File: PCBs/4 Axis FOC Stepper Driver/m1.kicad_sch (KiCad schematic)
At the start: 3 parts, among them J2 M1

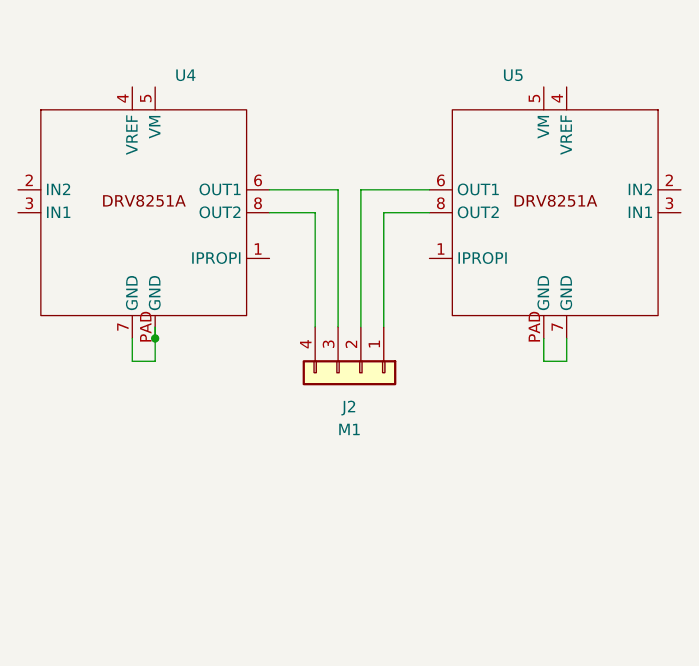
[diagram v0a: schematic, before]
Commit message: Start working on an integrated stepper driver
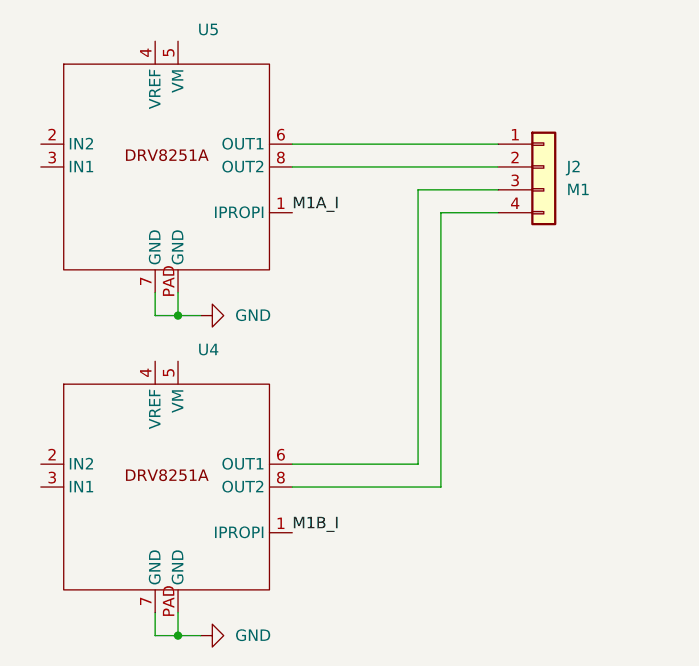
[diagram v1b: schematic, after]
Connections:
- net M1B_I: now reaches U4.1 (IPROPI)
- net GND: now reaches U4.7 (GND), U4.PAD (GND)
- net GND: now also U5.7 (GND), U5.PAD (GND)
- net at J2.1 (Pin_1): now also U5.6 (OUT1); no longer U5.8 (OUT2)
- net at J2.2 (Pin_2): now also U5.8 (OUT2); no longer U5.6 (OUT1)
- net M1A_I: now reaches U5.1 (IPROPI)
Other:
- moved on the sheet: J2, U4
